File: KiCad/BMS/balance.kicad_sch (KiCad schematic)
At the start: 127 parts, among them J5 430451000, Q1 PNP, Q10 NMOS, Q11 PNP, Q12 BSS138, Q13 NMOS, Q14 PNP, Q15 NMOS, Q16 PNP, Q17 NMOS, Q2 NMOS, Q3 PNP, Q4 NMOS, Q5 PNP, Q6 NMOS, Q7 PNP, Q8 NMOS, Q9 PNP, U10 TL431A, U11 MCP3201, U12 B0505MT, U13 TL431A, U14 HCPL-0630, U15 TL431A, U16 HCPL-0600, U17 TL431A, U18 HCPL-0600, U19 TL431A, U20 TL431A, U5 TL431A, U6 HCPL-0630, U7 74HC4051, U8 TL431A, U9 HCPL-0630

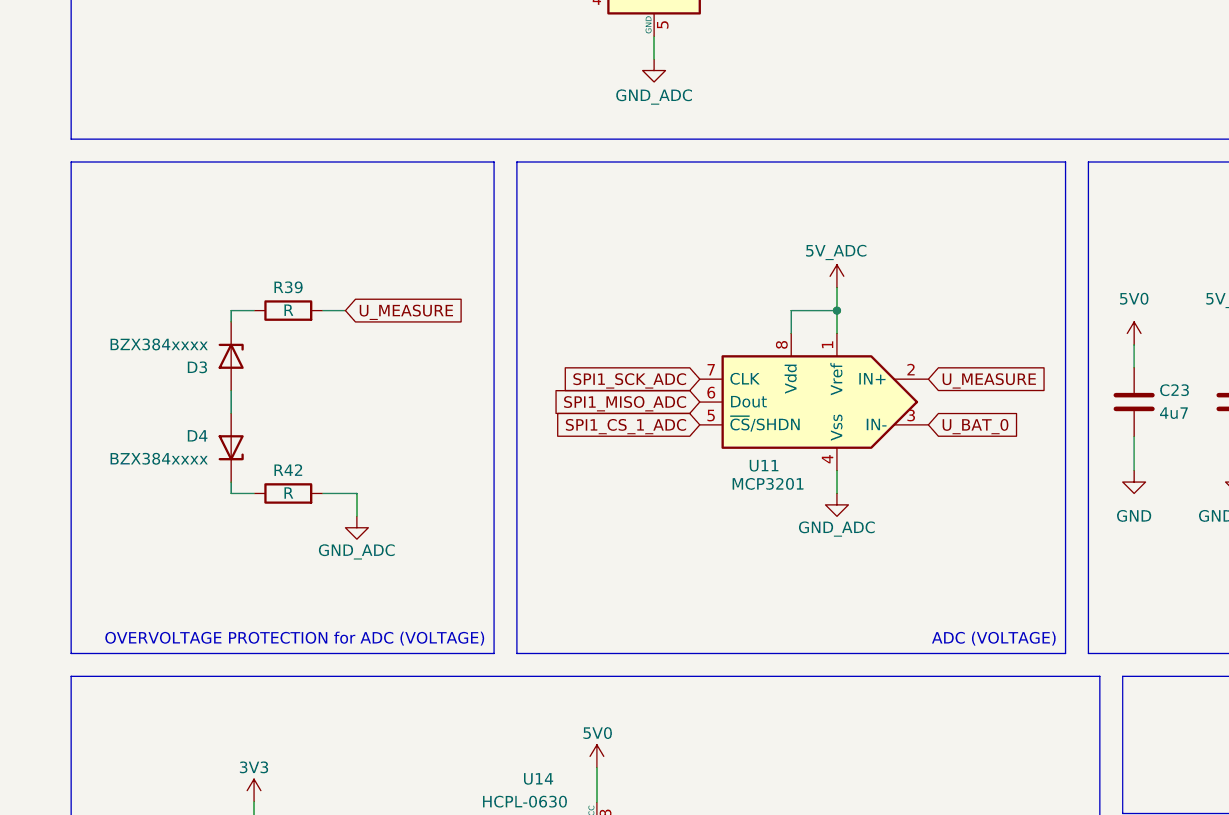
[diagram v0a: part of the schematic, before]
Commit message: 30.03.2025
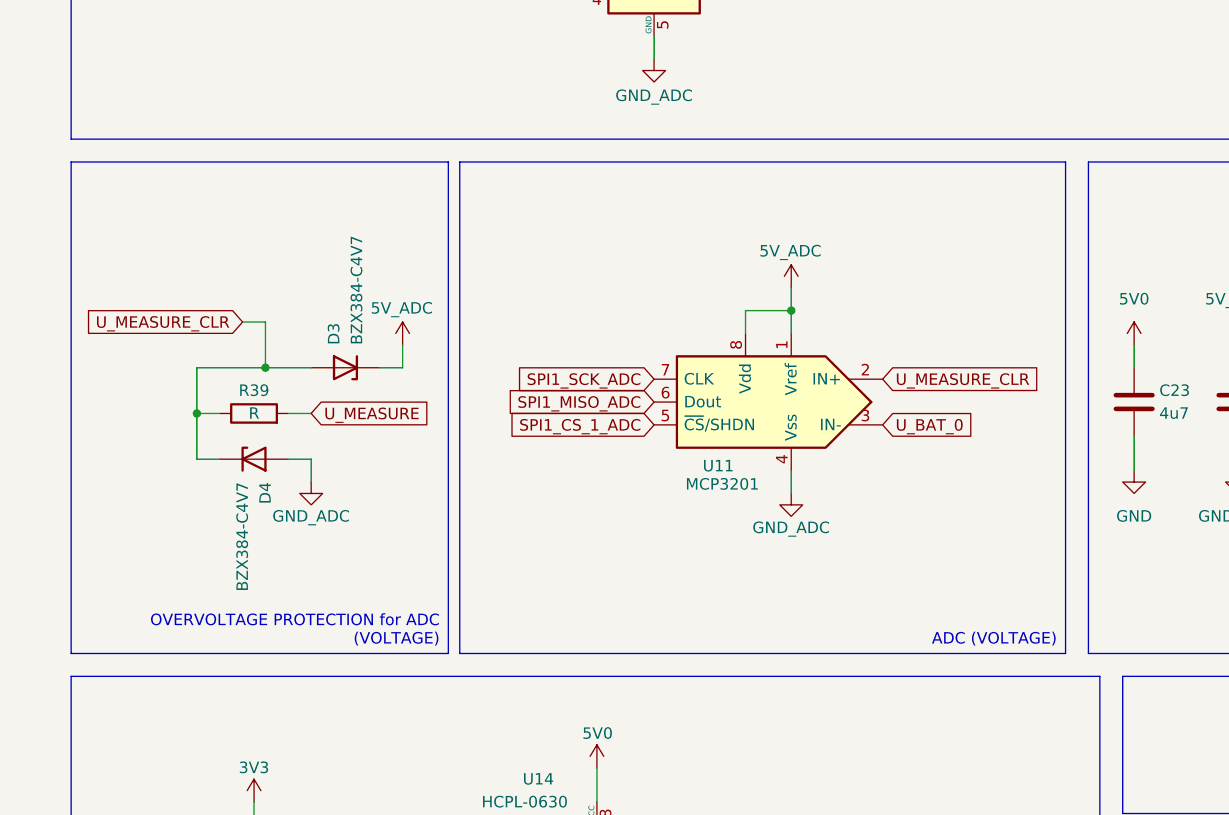
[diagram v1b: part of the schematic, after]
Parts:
- removed R42: R, Resistor_SMD:R_0603_1608Metric, symbol Device:R
- D3, D4: value BZX384xxxx -> BZX384-C4V7
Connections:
- net 5V_ADC: now also D3.1 (K)
- net GND_ADC: now also D4.2 (A)
- net U_MEASURE: no longer U11.2 (IN+)
- net U_MEASURE_CLR: now reaches D4.1 (K)
- net U_MEASURE_CLR: now also D3.2 (A), R39.1, U11.2 (IN+)
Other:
- moved on the sheet: D3, D4, R39, U11
